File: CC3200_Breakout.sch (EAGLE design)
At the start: 102 parts, among them J1 MJ-3536N, J22 M10X2, J23 M10X2, J3 SJ-3515-SMT, J4 SJ-3515-SMT, U1 TLV320AIC3254_RHB_32, U15 AT25FS010, U2 TPA2012D2_RTJ_20, Y2 32.768KHz, Y3 407MHz

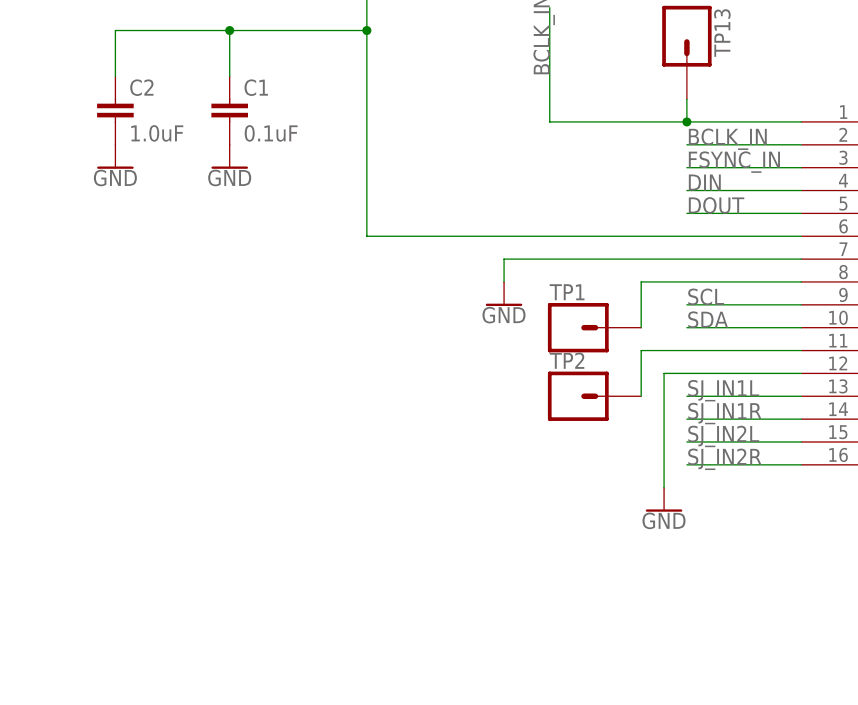
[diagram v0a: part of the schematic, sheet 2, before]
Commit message: routed
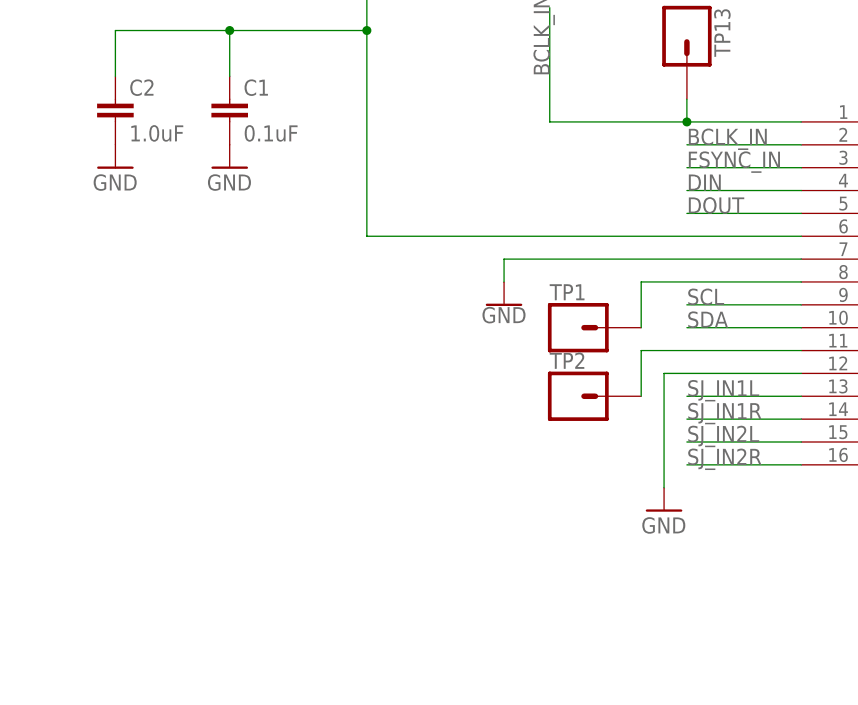
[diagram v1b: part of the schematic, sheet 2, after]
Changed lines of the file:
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@@
 <part name="C1" library="SparkFun-Capacitors" deviceset="0.1UF" device="-0402-16V-10%" value="0.1uF"/>
 <part name="C2" library="SparkFun-Capacitors" deviceset="1.0UF" device="-0402-16V-10%" value="1.0uF"/>
-<part name="GND33" library="SparkFun-PowerSymbols" deviceset="GND" device=""/>
-<part name="GND34" library="SparkFun-PowerSymbols" deviceset="GND" device=""/>
 <part name="GND35" library="SparkFun-PowerSymbols" deviceset="GND" device=""/>
 <part name="TP1" library="SparkFun-Connectors" deviceset="CONN_01" device=""/>
 <part name="TP2" library="SparkFun-Connectors" deviceset="CONN_01" device=""/>
-<part name="GND36" library="SparkFun-PowerSymbols" deviceset="GND" device=""/>
 <part name="GND37" library="SparkFun-PowerSymbols" deviceset="GND" device=""/>
 <part name="C3" library="SparkFun-Capacitors" deviceset="10UF" device="-0603-6.3V-20%" value="10uF"/>
@@
 <part name="R7" library="SparkFun-Resistors" deviceset="10KOHM" device="-0603-1/10W-1%" value="10k"/>
 <part name="SUPPLY7" library="SparkFun-Aesthetics" deviceset="3.3V" device=""/>
+<part name="GND64" library="SparkFun-Aesthetics" deviceset="GND" device=""/>
+<part name="GND33" library="SparkFun-Aesthetics" deviceset="GND" device=""/>
+<part name="GND34" library="SparkFun-Aesthetics" deviceset="GND" device=""/>
 </parts>
 <sheets>
@@
 <instance part="C1" gate="G$1" x="-114.3" y="149.86"/>
 <instance part="C2" gate="G$1" x="-127" y="149.86"/>
-<instance part="GND33" gate="1" x="-127" y="144.78"/>
-<instance part="GND34" gate="1" x="-114.3" y="144.78"/>
 <instance part="GND35" gate="1" x="-83.82" y="129.54"/>
 <instance part="TP1" gate="G$1" x="-76.2" y="127"/>
 <instance part="TP2" gate="G$1" x="-76.2" y="119.38"/>
-<instance part="GND36" gate="1" x="-66.04" y="106.68"/>
 <instance part="GND37" gate="1" x="35.56" y="104.14"/>
 <instance part="C3" gate="G$1" x="45.72" y="106.68"/>
@@
 <instance part="JMP1" gate="-0R" x="203.2" y="68.58"/>
 <instance part="JMP1" gate="G$2" x="200.66" y="71.12"/>
+<instance part="GND64" gate="1" x="-66.04" y="106.68"/>
+<instance part="GND33" gate="1" x="-114.3" y="144.78"/>
+<instance part="GND34" gate="1" x="-127" y="144.78"/>
 </instances>
 <busses>
@@
 <net name="GND" class="0">
 <segment>
-<pinref part="C2" gate="G$1" pin="2"/>
-<pinref part="GND33" gate="1" pin="GND"/>
-</segment>
-<segment>
-<pinref part="C1" gate="G$1" pin="2"/>
-<pinref part="GND34" gate="1" pin="GND"/>
-</segment>
-<segment>
 <pinref part="U1" gate="A" pin="OVISS"/>
 <wire x1="-50.8" y1="134.62" x2="-83.82" y2="134.62" width="0.1524" layer="91"/>
 <pinref part="GND35" gate="1" pin="GND"/>
 <wire x1="-83.82" y1="134.62" x2="-83.82" y2="132.08" width="0.1524" layer="91"/>
-</segment>
-<segment>
-<pinref part="GND36" gate="1" pin="GND"/>
-<wire x1="-66.04" y1="109.22" x2="-66.04" y2="121.92" width="0.1524" layer="91"/>
-<pinref part="U1" gate="A" pin="SPI_SELECT"/>
-<wire x1="-66.04" y1="121.92" x2="-50.8" y2="121.92" width="0.1524" layer="91"/>
 </segment>
 <segment>
@@
 <pinref part="GND62" gate="1" pin="GND"/>
 </segment>
-</net>
+<segment>
+<wire x1="-66.04" y1="109.22" x2="-66.04" y2="121.92" width="0.1524" layer="91"/>
+<pinref part="U1" gate="A" pin="SPI_SELECT"/>
+<wire x1="-66.04" y1="121.92" x2="-50.8" y2="121.92" width="0.1524" layer="91"/>
+<pinref part="GND64" gate="1" pin="GND"/>
+</segment>
+<segment>
+<pinref part="C1" gate="G$1" pin="2"/>
+<pinref part="GND33" gate="1" pin="GND"/>
+</segment>
+<segment>
+<pinref part="C2" gate="G$1" pin="2"/>
+<pinref part="GND34" gate="1" pin="GND"/>
+</segment>
+</net>
